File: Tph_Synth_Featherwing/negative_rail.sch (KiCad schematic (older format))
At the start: 5 parts

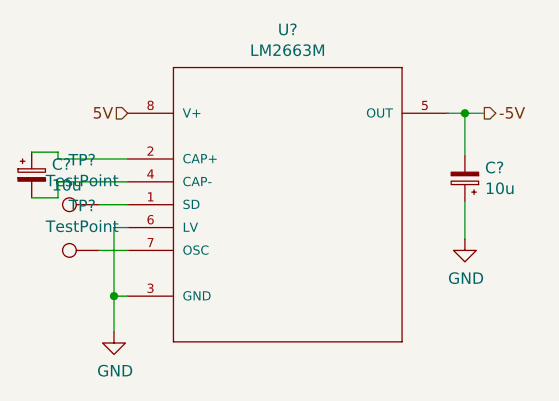
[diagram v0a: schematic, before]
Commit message: Added first-cut of schematic
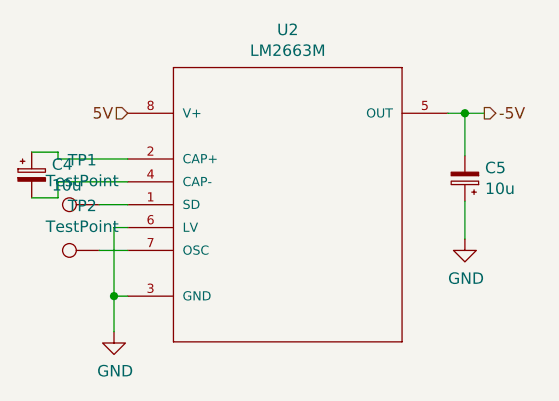
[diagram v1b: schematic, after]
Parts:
- gave numbers to parts that had none: 5
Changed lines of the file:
@@
 $EndDescr
 $Comp
-L LM2663M:LM2663M U?
+L LM2663M:LM2663M U2
 U 1 1 5DCC03A8
 P 5515 3250
-F 0 "U?" H 5515 3915 50  0000 C CNN
+F 0 "U2" H 5515 3915 50  0000 C CNN
 F 1 "LM2663M" H 5515 3824 50  0000 C CNN
 F 2 "SOIC127P620X175-8N" H 5515 3250 50  0001 L BNN
@@
 $EndBitmap
 $Comp
-L Device:CP_Small C?
+L Device:CP_Small C4
 U 1 1 5DECFC94
 P 4395 3220
-F 0 "C?" H 4483 3266 50  0000 L CNN
+F 0 "C4" H 4483 3266 50  0000 L CNN
 F 1 "10u" H 4483 3175 50  0000 L CNN
 F 2 "" H 4395 3220 50  0001 C CNN
@@
 $EndComp
 $Comp
-L Device:CP_Small C?
+L Device:CP_Small C5
 U 1 1 5DECFDD1
 P 6290 3235
-F 0 "C?" H 6202 3189 50  0000 R CNN
+F 0 "C5" H 6202 3189 50  0000 R CNN
 F 1 "10u" H 6202 3280 50  0000 R CNN
 F 2 "" H 6290 3235 50  0001 C CNN
@@
 $EndComp
 $Comp
-L Connector:TestPoint TP?
+L Connector:TestPoint TP2
 U 1 1 5DED0082
 P 4690 3550
-F 0 "TP?" V 4885 3624 50  0000 C CNN
+F 0 "TP2" V 4885 3624 50  0000 C CNN
 F 1 "TestPoint" V 4794 3624 50  0000 C CNN
 F 2 "" H 4890 3550 50  0001 C CNN
@@
 $EndComp
 $Comp
-L Connector:TestPoint TP?
+L Connector:TestPoint TP1
 U 1 1 5DED027A
 P 4690 3350
-F 0 "TP?" V 4885 3424 50  0000 C CNN
+F 0 "TP1" V 4885 3424 50  0000 C CNN
 F 1 "TestPoint" V 4794 3424 50  0000 C CNN
 F 2 "" H 4890 3350 50  0001 C CNN

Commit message: Initial attempt at PCB
Signed-off-by: Tisham Dhar <whatnickd@gmail.com>
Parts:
- C4, C5: footprint (none) -> Capacitor_SMD:C_0805_2012Metric
- TP1, TP2: footprint (none) -> TestPoint:TestPoint_Pad_D1.0mm
- U2: footprint SOIC127P620X175-8N -> Package_SO:SOIC-8_3.9x4.9mm_P1.27mm
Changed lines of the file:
@@
 F 0 "U2" H 5515 3915 50  0000 C CNN
 F 1 "LM2663M" H 5515 3824 50  0000 C CNN
-F 2 "SOIC127P620X175-8N" H 5515 3250 50  0001 L BNN
+F 2 "Package_SO:SOIC-8_3.9x4.9mm_P1.27mm" H 5515 3250 50  0001 L BNN
 F 3 "Unavailable" H 5515 3250 50  0001 L BNN
 F 4 "None" H 5515 3250 50  0001 L BNN "Field4"
@@
 F 0 "C4" H 4483 3266 50  0000 L CNN
 F 1 "10u" H 4483 3175 50  0000 L CNN
-F 2 "" H 4395 3220 50  0001 C CNN
+F 2 "Capacitor_SMD:C_0805_2012Metric" H 4395 3220 50  0001 C CNN
 F 3 "~" H 4395 3220 50  0001 C CNN
 	1    4395 3220
@@
 F 0 "C5" H 6202 3189 50  0000 R CNN
 F 1 "10u" H 6202 3280 50  0000 R CNN
-F 2 "" H 6290 3235 50  0001 C CNN
+F 2 "Capacitor_SMD:C_0805_2012Metric" H 6290 3235 50  0001 C CNN
 F 3 "~" H 6290 3235 50  0001 C CNN
 	1    6290 3235
@@
 F 0 "TP2" V 4885 3624 50  0000 C CNN
 F 1 "TestPoint" V 4794 3624 50  0000 C CNN
-F 2 "" H 4890 3550 50  0001 C CNN
+F 2 "TestPoint:TestPoint_Pad_D1.0mm" H 4890 3550 50  0001 C CNN
 F 3 "~" H 4890 3550 50  0001 C CNN
 	1    4690 3550
@@
 F 0 "TP1" V 4885 3424 50  0000 C CNN
 F 1 "TestPoint" V 4794 3424 50  0000 C CNN
-F 2 "" H 4890 3350 50  0001 C CNN
+F 2 "TestPoint:TestPoint_Pad_D1.0mm" H 4890 3350 50  0001 C CNN
 F 3 "~" H 4890 3350 50  0001 C CNN
 	1    4690 3350

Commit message: Added BOM and upgraded to kicad 5.0
Signed-off-by: Tisham Dhar <whatnickd@gmail.com>
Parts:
- C4, C5: manf# (none) -> GMK212BBJ106MG-T
- TP1, TP2: DNP (none) -> (none)
- U2: manf# (none) -> LM2663MX/NOPB
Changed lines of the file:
@@
 EESchema Schematic File Version 4
-LIBS:Tph_Synth_Featherwing-cache
-EELAYER 26 0
+EELAYER 30 0
 EELAYER END
 $Descr A4 11693 8268
@@
 F 7 "LM2663M" H 5515 3250 50  0001 L BNN "Field7"
 F 8 "Texas Instruments" H 5515 3250 50  0001 L BNN "Field8"
+F 9 "LM2663MX/NOPB" H 5515 3250 50  0001 C CNN "manf#"
 	1    5515 3250
 	1    0    0    -1
@@
 F 2 "Capacitor_SMD:C_0805_2012Metric" H 4395 3220 50  0001 C CNN
 F 3 "~" H 4395 3220 50  0001 C CNN
+F 4 "GMK212BBJ106MG-T" H 4395 3220 50  0001 C CNN "manf#"
 	1    4395 3220
 	1    0    0    -1
@@
 F 2 "Capacitor_SMD:C_0805_2012Metric" H 6290 3235 50  0001 C CNN
 F 3 "~" H 6290 3235 50  0001 C CNN
+F 4 "GMK212BBJ106MG-T" H 6290 3235 50  0001 C CNN "manf#"
 	1    6290 3235
 	-1   0    0    1
@@
 F 2 "TestPoint:TestPoint_Pad_D1.0mm" H 4890 3550 50  0001 C CNN
 F 3 "~" H 4890 3550 50  0001 C CNN
+F 4 " " H 4690 3550 50  0001 C CNN "DNP"
 	1    4690 3550
 	0    -1   -1   0
@@
 F 2 "TestPoint:TestPoint_Pad_D1.0mm" H 4890 3350 50  0001 C CNN
 F 3 "~" H 4890 3350 50  0001 C CNN
+F 4 " " H 4690 3350 50  0001 C CNN "DNP"
 	1    4690 3350
 	0    -1   -1   0
